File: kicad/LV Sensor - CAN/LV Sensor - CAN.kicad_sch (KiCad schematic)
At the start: 9 parts, among them J2 Conn_01x09_Pin, U1 MCP2518FD-xJHA, U2 DSC1001DL5-020.0000T, U5 ATA6561-GAQW-N

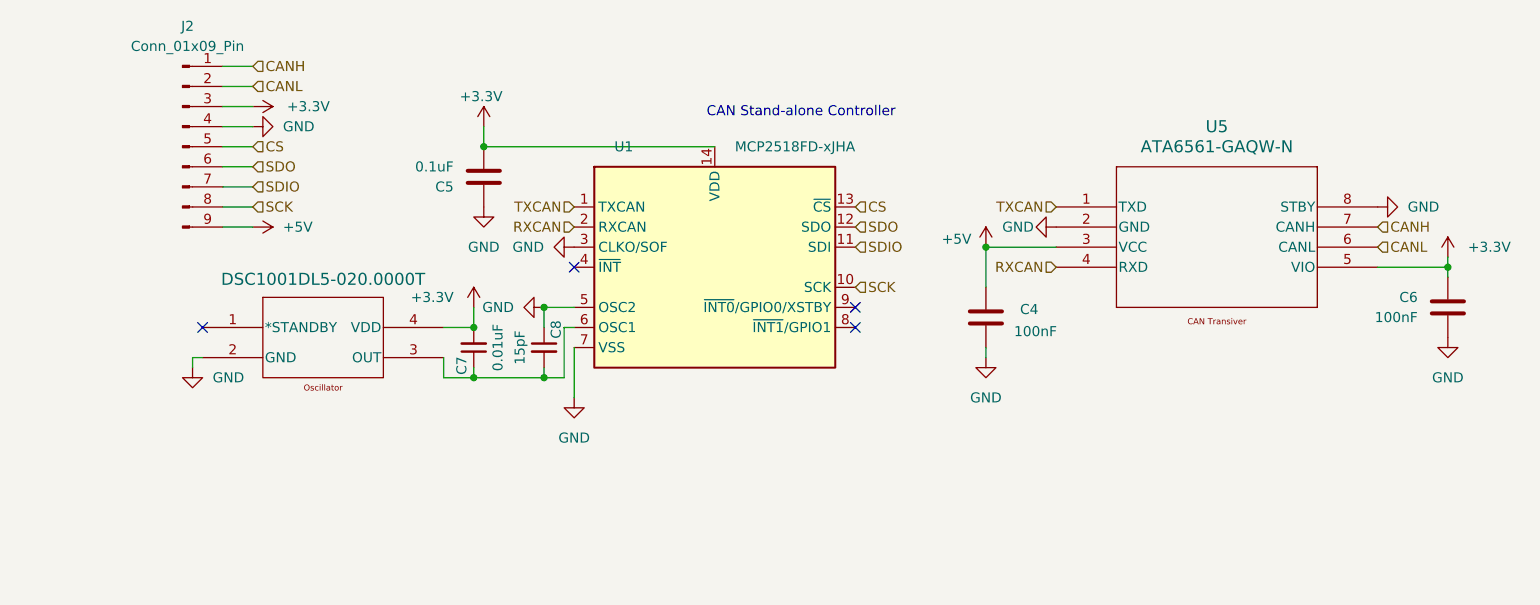
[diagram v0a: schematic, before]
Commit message: work faster 🍘
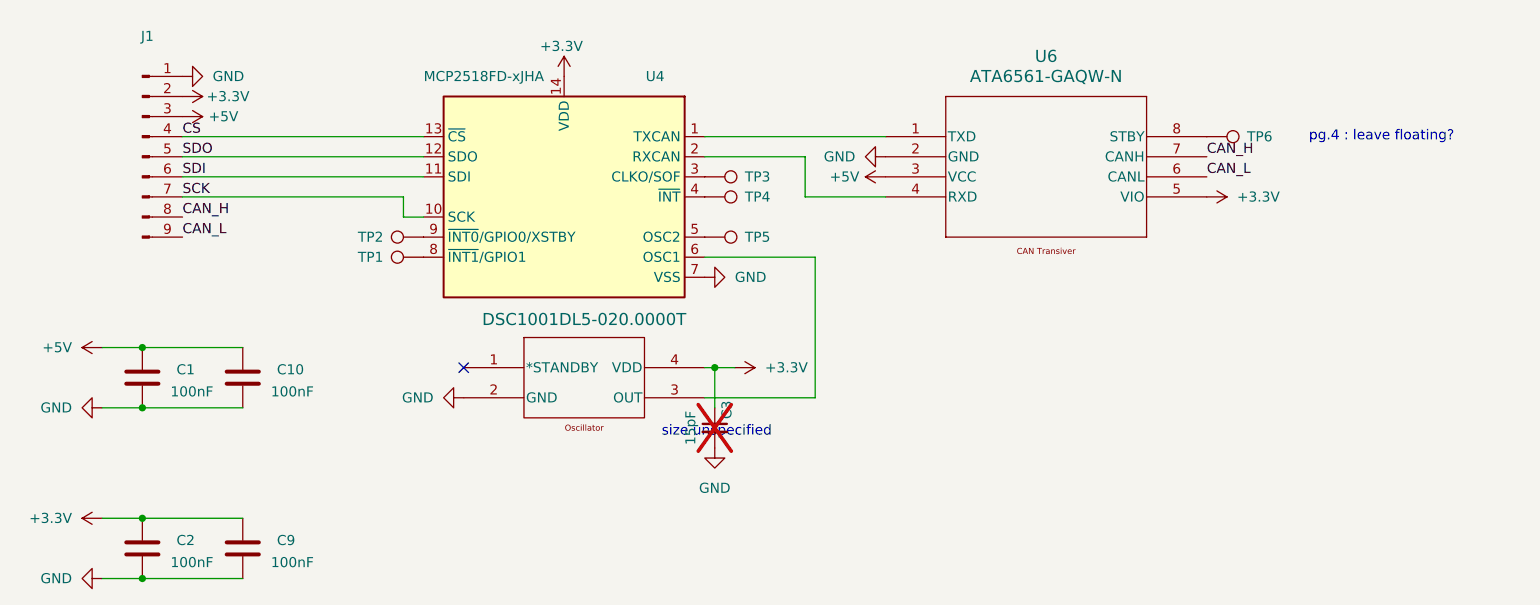
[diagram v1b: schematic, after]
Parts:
- removed C4, C6: 100nF, Capacitor_SMD:C_1206_3216Metric_Pad1.33x1.80mm_HandSolder, symbol Device:C
- removed C5: 0.1uF, Capacitor_SMD:C_1206_3216Metric_Pad1.33x1.80mm_HandSolder, symbol Device:C
- removed C7: 0.01uF, Capacitor_SMD:C_1206_3216Metric_Pad1.33x1.80mm_HandSolder, symbol Device:C_Small
- removed C8: 15pF, Capacitor_SMD:C_1206_3216Metric_Pad1.33x1.80mm_HandSolder, symbol Device:C_Small
- removed J2: Conn_01x09_Pin, Connector_PinHeader_2.54mm:PinHeader_1x09_P2.54mm_Vertical, symbol Connector:Conn_01x09_Pin
- removed U1: MCP2518FD-xJHA, LV-Sensor-Footprints-Lib:MCP2518FDT, symbol LV-Sensor-Lib:MCP2517FD-xJHA
- removed U2: DSC1001DL5-020.0000T, LV-Sensor-Footprints-Lib:CDFN4_2P5X2_MCH, symbol LV-Sensor-Lib:DSC1001DL5-020.0000T
- removed U5: ATA6561-GAQW-N, LV-Sensor-Footprints-Lib:SOIC8_4P9X3P9MC_MCH, symbol LV-Sensor-Lib:ATA6561-GAQW-N
- added C1, C10, C2, C9: 100nF, Capacitor_SMD:C_1206_3216Metric_Pad1.33x1.80mm_HandSolder, symbol Device:C
- added C3: 15pF, Capacitor_SMD:C_1206_3216Metric_Pad1.33x1.80mm_HandSolder, symbol Device:C_Small
- added J1: Conn_01x09_Pin, Connector_PinHeader_2.54mm:PinHeader_1x09_P2.54mm_Vertical, symbol Connector:Conn_01x09_Pin
- added TP1, TP2, TP3, TP4, TP5, TP6: TestPoint, Connector_Pin:Pin_D1.0mm_L10.0mm, symbol Connector:TestPoint
- added U3: DSC1001DL5-020.0000T, LV-Sensor-Footprints-Lib:CDFN4_2P5X2_MCH, symbol LV-Sensor-Lib:DSC1001DL5-020.0000T
- added U4: MCP2518FD-xJHA, LV-Sensor-Footprints-Lib:MCP2518FDT, symbol LV-Sensor-Lib:MCP2517FD-xJHA
- added U6: ATA6561-GAQW-N, LV-Sensor-Footprints-Lib:SOIC8_4P9X3P9MC_MCH, symbol LV-Sensor-Lib:ATA6561-GAQW-N
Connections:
- net +3.3V: now also C2.1, C3.1, C9.1, J1.2 (Pin_2), U3.4 (VDD), U4.14 (VDD), U6.5 (VIO)
- net +5V: now also C1.1, C10.1, J1.3 (Pin_3), U6.3 (VCC)
- net CS: now also J1.4 (Pin_4), U4.13 (~{CS})
- net GND: now also C1.2, C10.2, C2.2, C3.2, C9.2, J1.1 (Pin_1), U3.2 (GND), U4.7 (VSS), U6.2 (GND)
- net SCK: now also J1.7 (Pin_7), U4.10 (SCK)
- net SDO: now also J1.5 (Pin_5), U4.12 (SDO)
- new net: U3.3 (OUT), U4.6 (OSC1)
- new net: U4.1 (TXCAN), U6.1 (TXD)
- new net: U4.2 (RXCAN), U6.4 (RXD)
- new net: TP3.1, U4.3 (CLKO/SOF)
- new net: TP4.1, U4.4 (~{INT})
- new net: TP5.1, U4.5 (OSC2)
- new net: TP1.1, U4.8 (~{INT1}/GPIO1)
- new net: TP2.1, U4.9 (~{INT0}/GPIO0/XSTBY)
- new net: TP6.1, U6.8 (STBY)
- new net CAN_H: J1.8 (Pin_8), U6.7 (CANH)
- new net CAN_L: J1.9 (Pin_9), U6.6 (CANL)
- new net SDI: J1.6 (Pin_6), U4.11 (SDI)
- no-connect marks 4 -> 1
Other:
- note added: "pg.4 : leave floating?"
- note added: "size unspecified"
- note removed: "CAN Stand-alone Controller"
